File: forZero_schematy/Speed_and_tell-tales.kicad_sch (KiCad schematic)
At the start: 32 parts, among them Q10 AO3400A, Q3 AO3400A, Q4 AO3400A, Q5 AO3400A, Q6 AO3400A, Q7 AO3400A, Q8 AO3400A, Q9 AO3400A

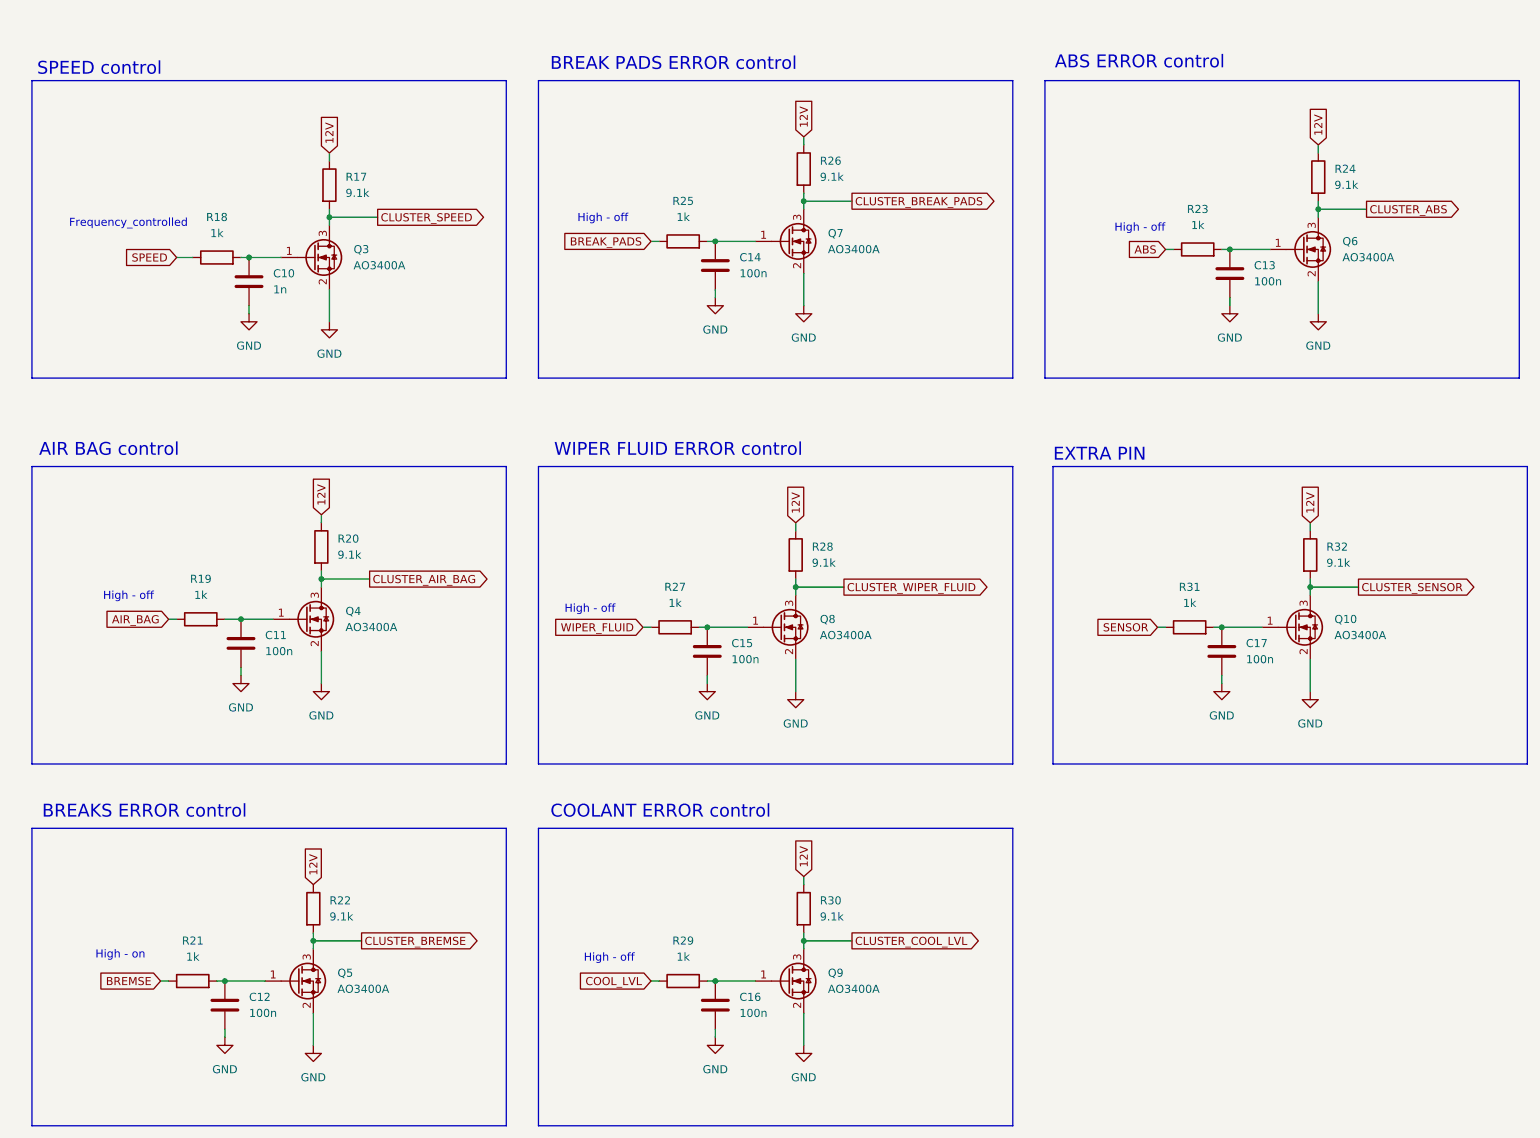
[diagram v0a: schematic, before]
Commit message: Wprowadzenie poprawek PCB
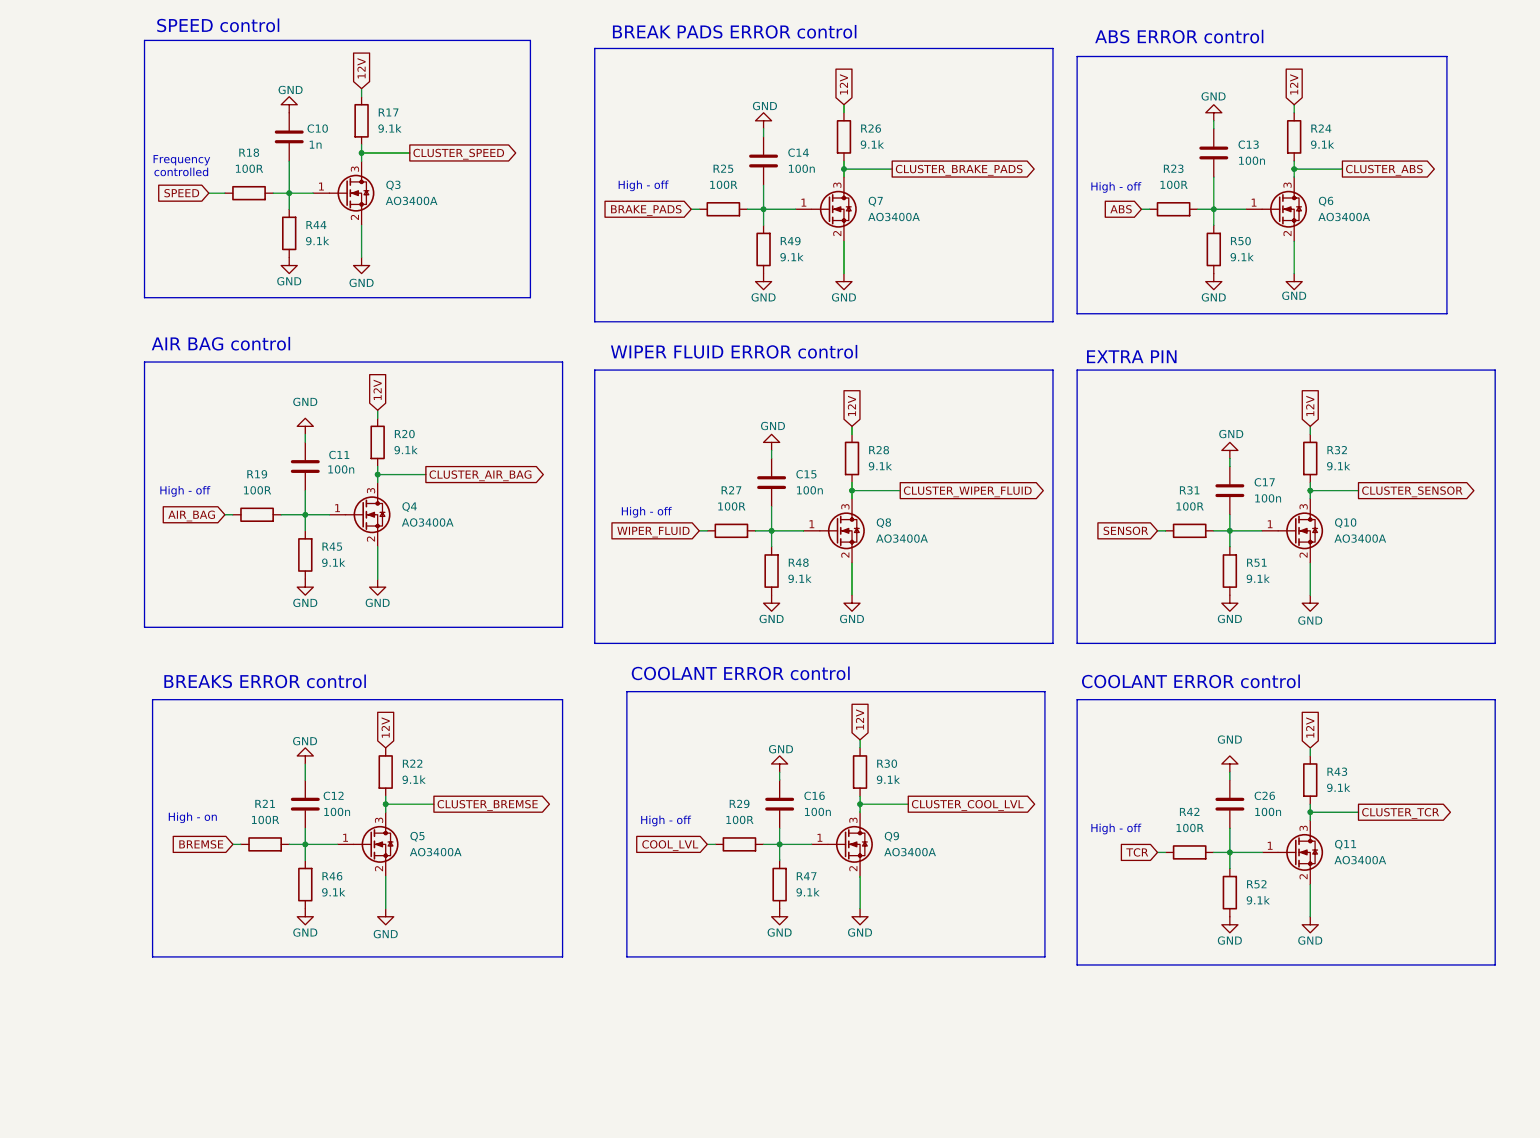
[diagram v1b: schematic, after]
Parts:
- added C26: 100n, Capacitor_SMD:C_0805_2012Metric_Pad1.18x1.45mm_HandSolder, symbol Device:C
- added Q11: AO3400A, Package_TO_SOT_SMD:SOT-23, symbol Transistor_FET:AO3400A
- added R42: 100R, Resistor_SMD:R_0805_2012Metric_Pad1.20x1.40mm_HandSolder, symbol Device:R
- added R43, R44, R45, R46, R47, R48, R49, R50, R51, R52: 9.1k, Resistor_SMD:R_0805_2012Metric_Pad1.20x1.40mm_HandSolder, symbol Device:R
- R18, R19, R21, R23, R25, R27, R29, R31: value 1k -> 100R
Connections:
- net 12V: now also R43.1
- net GND: now also C10.1, C12.1, C13.1, C14.1, C15.1, C16.1, C17.1, C26.1, Q11.2 (S), R44.1, R45.1, R46.1, R47.1, R48.1, R49.1, R50.1, R51.1, R52.1; no longer C10.2, C12.2, C13.2, C14.2, C15.2, C16.2, C17.2
- net at Q5.1 (G), R21.2: now also C12.2, R46.2; no longer C12.1
- net at Q10.1 (G), R31.2: now also C17.2, R51.2; no longer C17.1
- net at Q3.1 (G), R18.2: now also C10.2, R44.2; no longer C10.1
- net at Q6.1 (G), R23.2: now also C13.2, R50.2; no longer C13.1
- net at Q7.1 (G), R25.2: now also C14.2, R49.2; no longer C14.1
- net at Q8.1 (G), R27.2: now also C15.2, R48.2; no longer C15.1
- net at Q9.1 (G), R29.2: now also C16.2, R47.2; no longer C16.1
- net at C11.1, Q4.1 (G), R19.2: now also R45.2
- net BREAK_PADS renamed BRAKE_PADS
- net CLUSTER_BREAK_PADS renamed CLUSTER_BRAKE_PADS
- new net: C26.2, Q11.1 (G), R42.2, R52.2
- new net CLUSTER_TCR: Q11.3 (D), R43.2
- new net TCR: R42.1
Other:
- note added: "Frequency controlled"
- note removed: "Frequency_controlled"
- moved on the sheet: C10, C11, C12, C13, C14, C15, C16, C17, Q10, Q3, Q4, Q5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
